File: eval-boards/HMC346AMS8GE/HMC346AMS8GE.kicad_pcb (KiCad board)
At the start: 2 copper layers, 8 parts, among them J1 Conn_Coaxial, J2 Conn_Coaxial, J3 Conn_01x04_Male, U1 HMC346AMS8GE

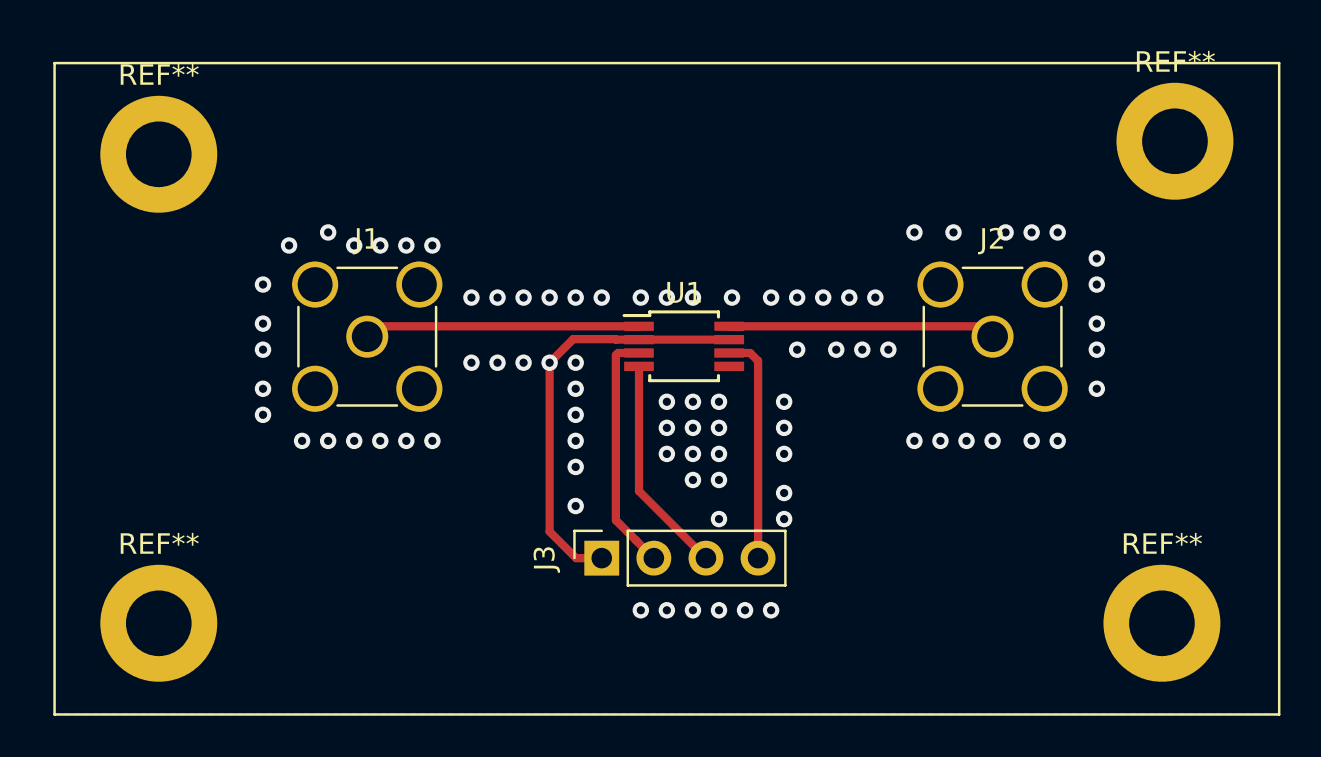
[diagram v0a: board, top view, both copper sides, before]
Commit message: final vision
最终版
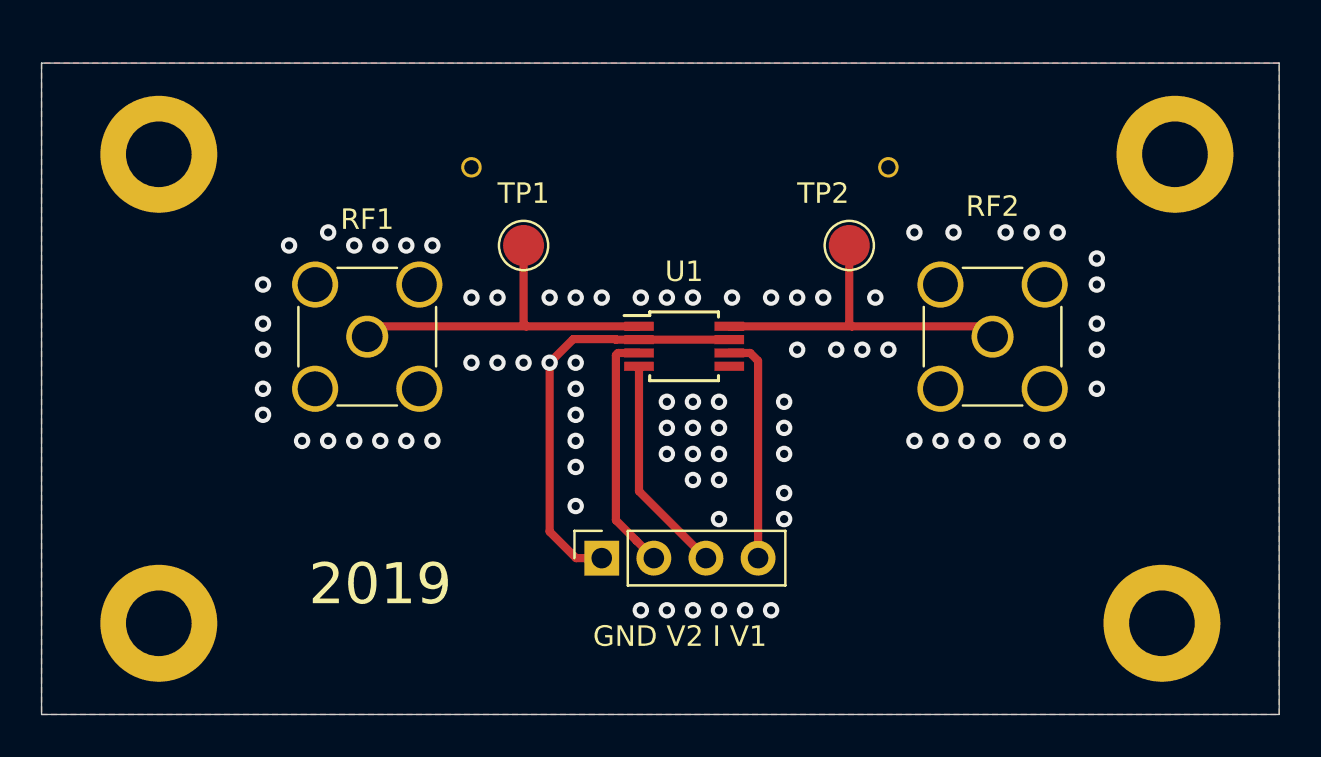
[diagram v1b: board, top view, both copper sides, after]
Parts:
- added REF**: PinSocket_1x01_P1.27mm_Vertical, Connector_PinSocket_1.27mm:PinSocket_1x01_P1.27mm_Vertical, F.Cu at (121.9, 110.5)
- added REF**: PinSocket_1x01_P1.27mm_Vertical, Connector_PinSocket_1.27mm:PinSocket_1x01_P1.27mm_Vertical, F.Cu at (142.2, 110.5)
- added TP1: TestPoint_Pad_D2.0mm, TestPoint:TestPoint_Pad_D2.0mm, F.Cu at (124.5, 114.3)
- added TP2: TestPoint_Pad_D2.0mm, TestPoint:TestPoint_Pad_D2.0mm, F.Cu at (140.3, 114.3)
- GND V2 I V1: renamed from J3
- moved REF** 0.64 mm to (156.2, 109.9)
- renumbered J1 to RF1, J2 to RF2
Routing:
- net Net-(J1-Pad1): track 13.5 -> 17.4 mm
- net Net-(J2-Pad1): track 13.0 -> 17.0 mm
- net GND: vias 85 -> 83
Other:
- board outline added: 60.3 x 31.8 mm
- board text added: "2019"
